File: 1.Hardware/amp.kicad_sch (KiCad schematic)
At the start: 6 parts, among them U2 MAX98357A

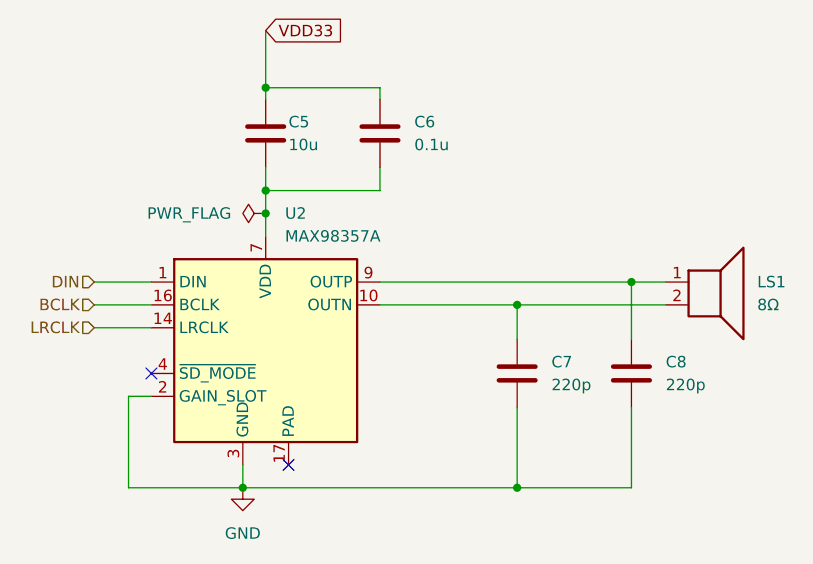
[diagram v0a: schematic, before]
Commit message: ready for routing/placement
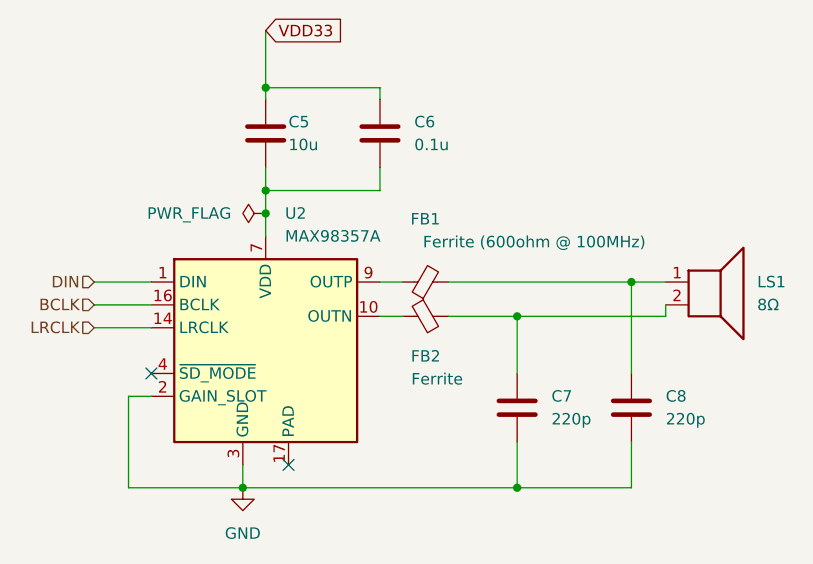
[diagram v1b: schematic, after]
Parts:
- added FB1: Ferrite (600ohm @ 100MHz), BLM21:BEADC2012X105N, symbol Device:FerriteBead_Small
- added FB2: Ferrite, BLM21:BEADC2012X105N, symbol Device:FerriteBead_Small
- C5, C6, C7, C8: footprint (none) -> Capacitor_SMD:C_0603_1608Metric_Pad1.08x0.95mm_HandSolder
- LS1: footprint (none) -> TerminalBlock_Phoenix:TerminalBlock_Phoenix_MPT-0,5-2-2.54_1x02_P2.54mm_Horizontal
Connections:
- net at C7.1, LS1.2: now also FB2.2; no longer U2.10 (OUTN)
- net at C8.1, LS1.1: now also FB1.2; no longer U2.9 (OUTP)
- new net: FB2.1, U2.10 (OUTN)
- new net: FB1.1, U2.9 (OUTP)
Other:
- moved on the sheet: C7, C8
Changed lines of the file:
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@@
-	)
-	(junction
-		(at 165.1 81.28)
-		(diameter 0)
-		(color 0 0 0 0)
 	)
 	(junction
@@
 	)
 	(junction
+		(at 165.1 82.55)
+		(diameter 0)
+		(color 0 0 0 0)
+	)
+	(junction
 		(at 137.16 71.12)
+		(diameter 0)
+		(color 0 0 0 0)
+	)
+	(junction
+		(at 165.1 101.6)
 		(diameter 0)
 		(color 0 0 0 0)
@@
 	)
 	(junction
-		(at 165.1 101.6)
-		(diameter 0)
-		(color 0 0 0 0)
-	)
-	(junction
 		(at 134.62 101.6)
 		(diameter 0)
@@
 	(wire
 		(pts
-			(xy 165.1 92.71) (xy 165.1 101.6)
+			(xy 181.61 82.55) (xy 181.61 81.28)
+		)
+		(stroke
+			(width 0)
+			(type default)
+		)
+	)
+	(wire
+		(pts
+			(xy 165.1 96.52) (xy 165.1 101.6)
 		)
 		(stroke
@@
 	(wire
 		(pts
-			(xy 165.1 81.28) (xy 181.61 81.28)
-		)
-		(stroke
-			(width 0)
-			(type default)
-		)
-	)
-	(wire
-		(pts
-			(xy 149.86 78.74) (xy 177.8 78.74)
+			(xy 165.1 82.55) (xy 181.61 82.55)
+		)
+		(stroke
+			(width 0)
+			(type default)
+		)
+	)
+	(wire
+		(pts
+			(xy 157.48 78.74) (xy 177.8 78.74)
 		)
 		(stroke
@@
 	(wire
 		(pts
-			(xy 177.8 92.71) (xy 177.8 101.6)
+			(xy 177.8 96.52) (xy 177.8 101.6)
+		)
+		(stroke
+			(width 0)
+			(type default)
+		)
+	)
+	(wire
+		(pts
+			(xy 149.86 78.74) (xy 152.4 78.74)
 		)
 		(stroke
@@
 	(wire
 		(pts
-			(xy 149.86 81.28) (xy 165.1 81.28)
-		)
-		(stroke
-			(width 0)
-			(type default)
-		)
-	)
-	(wire
-		(pts
 			(xy 118.11 83.82) (xy 124.46 83.82)
 		)
@@
 	(wire
 		(pts
-			(xy 177.8 78.74) (xy 177.8 85.09)
+			(xy 149.86 82.55) (xy 152.4 82.55)
+		)
+		(stroke
+			(width 0)
+			(type default)
+		)
+	)
+	(wire
+		(pts
+			(xy 177.8 78.74) (xy 177.8 88.9)
 		)
 		(stroke
@@
 	(wire
 		(pts
-			(xy 165.1 81.28) (xy 165.1 85.09)
+			(xy 165.1 82.55) (xy 165.1 88.9)
+		)
+		(stroke
+			(width 0)
+			(type default)
+		)
+	)
+	(wire
+		(pts
+			(xy 157.48 82.55) (xy 165.1 82.55)
 		)
 		(stroke
@@
 	)
 	(symbol
+		(lib_id "Device:FerriteBead_Small")
+		(at 154.94 82.55 90)
+		(mirror x)
+		(unit 1)
+		(exclude_from_sim no)
+		(in_bom yes)
+		(on_board yes)
+		(dnp no)
+		(property "Reference" "FB2"
+			(at 154.94 86.995 90)
+			(effects
+				(font
+					(size 1.27 1.27)
+				)
+			)
+		)
+		(property "Value" "Ferrite"
+			(at 156.21 89.535 90)
+			(effects
+				(font
+					(size 1.27 1.27)
+				)
+			)
+		)
+		(property "Footprint" "BLM21:BEADC2012X105N"
+			(at 154.94 80.772 90)
+			(effects
+				(font
+					(size 1.27 1.27)
+				)
+				(hide yes)
+			)
+		)
+		(property "Datasheet" "~"
+			(at 154.94 82.55 0)
+			(effects
+				(font
+					(size 1.27 1.27)
+				)
+				(hide yes)
+			)
+		)
+		(property "Description" "Ferrite bead, small symbol"
+			(at 154.94 82.55 0)
+			(effects
+				(font
+					(size 1.27 1.27)
+				)
+				(hide yes)
+			)
+		)
+		(pin "1"
+		)
+		(pin "2"
+		)
+		(instances
+			(project "jukebox"
+				(path "/d400bd10-35e9-4717-b347-ccb991be6072/58aa8eb1-6419-4649-9641-e1795f62a7f1"
+					(reference "FB2")
+					(unit 1)
+				)
+			)
+		)
+	)
+	(symbol
 		(lib_id "Device:C")
-		(at 165.1 88.9 0)
+		(at 165.1 92.71 0)
 		(unit 1)
 		(exclude_from_sim no)
@@
 		(fields_autoplaced yes)
 		(property "Reference" "C7"
-			(at 168.91 87.6299 0)
+			(at 168.91 91.4399 0)
 			(effects
 				(font
@@
 		)
 		(property "Value" "220p"
-			(at 168.91 90.1699 0)
-			(effects
-				(font
-					(size 1.27 1.27)
-				)
-				(justify left)
-			)
-		)
-		(property "Footprint" ""
-			(at 166.0652 92.71 0)
+			(at 168.91 93.9799 0)
+			(effects
+				(font
+					(size 1.27 1.27)
+				)
+				(justify left)
+			)
+		)
+		(property "Footprint" "Capacitor_SMD:C_0603_1608Metric_Pad1.08x0.95mm_HandSolder"
+			(at 166.0652 96.52 0)
 			(effects
 				(font
@@
 		)
 		(property "Datasheet" "~"
-			(at 165.1 88.9 0)
+			(at 165.1 92.71 0)
 			(effects
 				(font
@@
 		)
 		(property "Description" "Unpolarized capacitor"
-			(at 165.1 88.9 0)
+			(at 165.1 92.71 0)
 			(effects
 				(font
@@
 			)
 		)
-		(property "Footprint" ""
+		(property "Footprint" "TerminalBlock_Phoenix:TerminalBlock_Phoenix_MPT-0,5-2-2.54_1x02_P2.54mm_Horizontal"
 			(at 186.69 83.82 0)
 			(effects
@@
 	(symbol
 		(lib_id "Device:C")
-		(at 177.8 88.9 0)
+		(at 177.8 92.71 0)
 		(unit 1)
 		(exclude_from_sim no)
@@
 		(fields_autoplaced yes)
 		(property "Reference" "C8"
-			(at 181.61 87.6299 0)
+			(at 181.61 91.4399 0)
 			(effects
 				(font
@@
 		)
 		(property "Value" "220p"
-			(at 181.61 90.1699 0)
-			(effects
-				(font
-					(size 1.27 1.27)
-				)
-				(justify left)
-			)
-		)
-		(property "Footprint" ""
-			(at 178.7652 92.71 0)
+			(at 181.61 93.9799 0)
+			(effects
+				(font
+					(size 1.27 1.27)
+				)
+				(justify left)
+			)
+		)
+		(property "Footprint" "Capacitor_SMD:C_0603_1608Metric_Pad1.08x0.95mm_HandSolder"
+			(at 178.7652 96.52 0)
 			(effects
 				(font
@@
 		)
 		(property "Datasheet" "~"
-			(at 177.8 88.9 0)
+			(at 177.8 92.71 0)
 			(effects
 				(font
@@
 		)
 		(property "Description" "Unpolarized capacitor"
-			(at 177.8 88.9 0)
+			(at 177.8 92.71 0)
 			(effects
 				(font
@@
 			)
 		)
-		(property "Footprint" ""
+		(property "Footprint" "Capacitor_SMD:C_0603_1608Metric_Pad1.08x0.95mm_HandSolder"
 			(at 138.1252 66.04 0)
 			(effects
@@
 				(path "/d400bd10-35e9-4717-b347-ccb991be6072/58aa8eb1-6419-4649-9641-e1795f62a7f1"
 					(reference "C5")
+					(unit 1)
+				)
+			)
+		)
+	)
+	(symbol
+		(lib_id "Device:FerriteBead_Small")
+		(at 154.94 78.74 90)
+		(unit 1)
+		(exclude_from_sim no)
+		(in_bom yes)
+		(on_board yes)
+		(dnp no)
+		(property "Reference" "FB1"
+			(at 154.9019 71.755 90)
+			(effects
+				(font
+					(size 1.27 1.27)
+				)
+			)
+		)
+		(property "Value" "Ferrite (600ohm @ 100MHz)"
+			(at 167.005 74.295 90)
+			(effects
+				(font
+					(size 1.27 1.27)
+				)
+			)
+		)
+		(property "Footprint" "BLM21:BEADC2012X105N"
+			(at 154.94 80.518 90)
+			(effects
+				(font
+					(size 1.27 1.27)
+				)
+				(hide yes)
+			)
+		)
+		(property "Datasheet" "~"
+			(at 154.94 78.74 0)
+			(effects
+				(font
+					(size 1.27 1.27)
+				)
+				(hide yes)
+			)
+		)
+		(property "Description" "Ferrite bead, small symbol"
+			(at 154.94 78.74 0)
+			(effects
+				(font
+					(size 1.27 1.27)
+				)
+				(hide yes)
+			)
+		)
+		(property "Purpose" ""
+			(at 154.94 78.74 0)
+			(effects
+				(font
+					(size 1.27 1.27)
+				)
+			)
+		)
+		(pin "1"
+		)
+		(pin "2"
+		)
+		(instances
+			(project ""
+				(path "/d400bd10-35e9-4717-b347-ccb991be6072/58aa8eb1-6419-4649-9641-e1795f62a7f1"
+					(reference "FB1")
 					(unit 1)
 				)
@@
 			)
 		)
+		(property "Purpose" ""
+			(at 137.16 86.36 0)
+			(effects
+				(font
+					(size 1.27 1.27)
+				)
+			)
+		)
 		(pin "6"
 		)
@@
 			)
 		)
-		(property "Footprint" ""
+		(property "Footprint" "Capacitor_SMD:C_0603_1608Metric_Pad1.08x0.95mm_HandSolder"
 			(at 150.8252 66.04 0)
 			(effects
